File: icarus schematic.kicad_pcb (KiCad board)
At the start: 2 copper layers, 40 x 60 mm, 58 parts, among them J1 Conn_01x02_Socket, J2 USB_C_Receptacle_USB2.0_16P, J3 Conn_01x02_Socket, J4 Conn_01x02_Socket, J5 Conn_01x02_Socket, Q1 AO3400A, Q2 AO3400A, Q3 AO3400A, Q4 AO3400A, SW1 SW_Push(BOOt), SW2 SW_Push(EN), U2 BMI088, U3 AMS1117-3.3, U4 ESP32-S3-WROOM-1

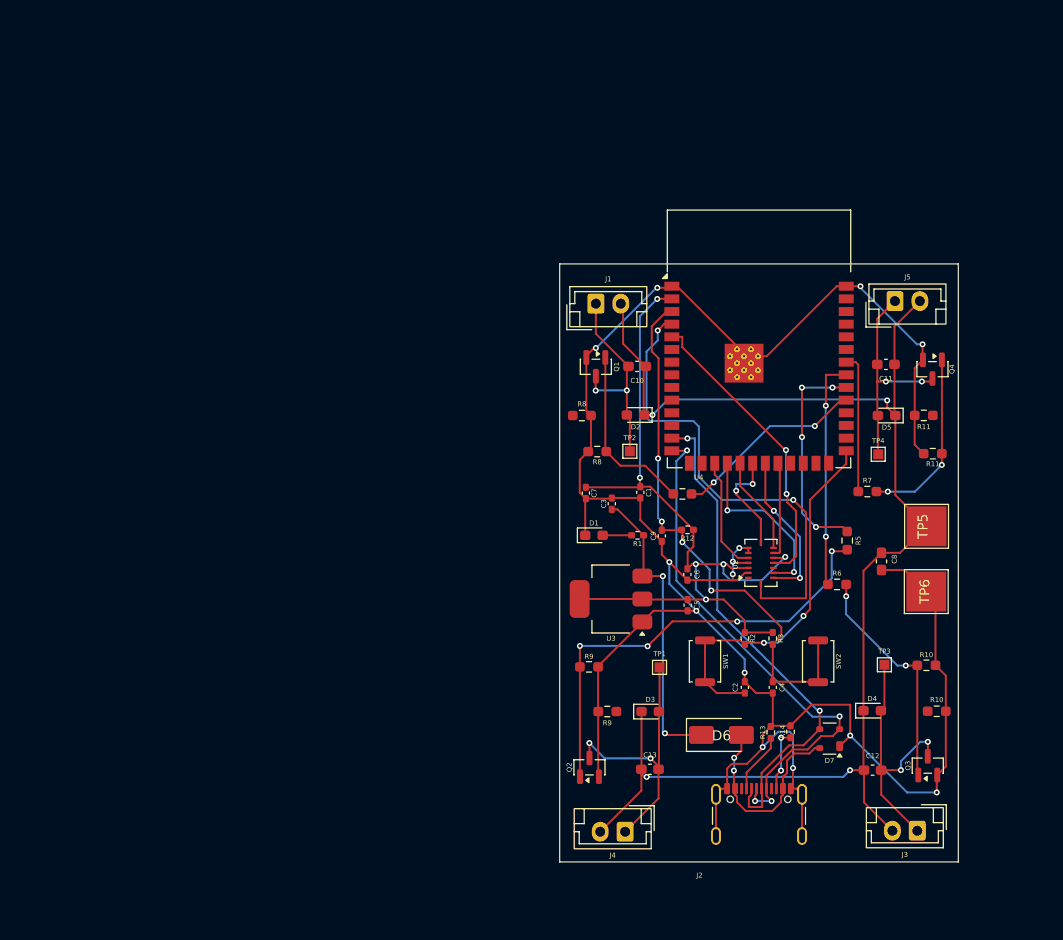
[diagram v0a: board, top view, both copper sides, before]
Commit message: Add files via upload
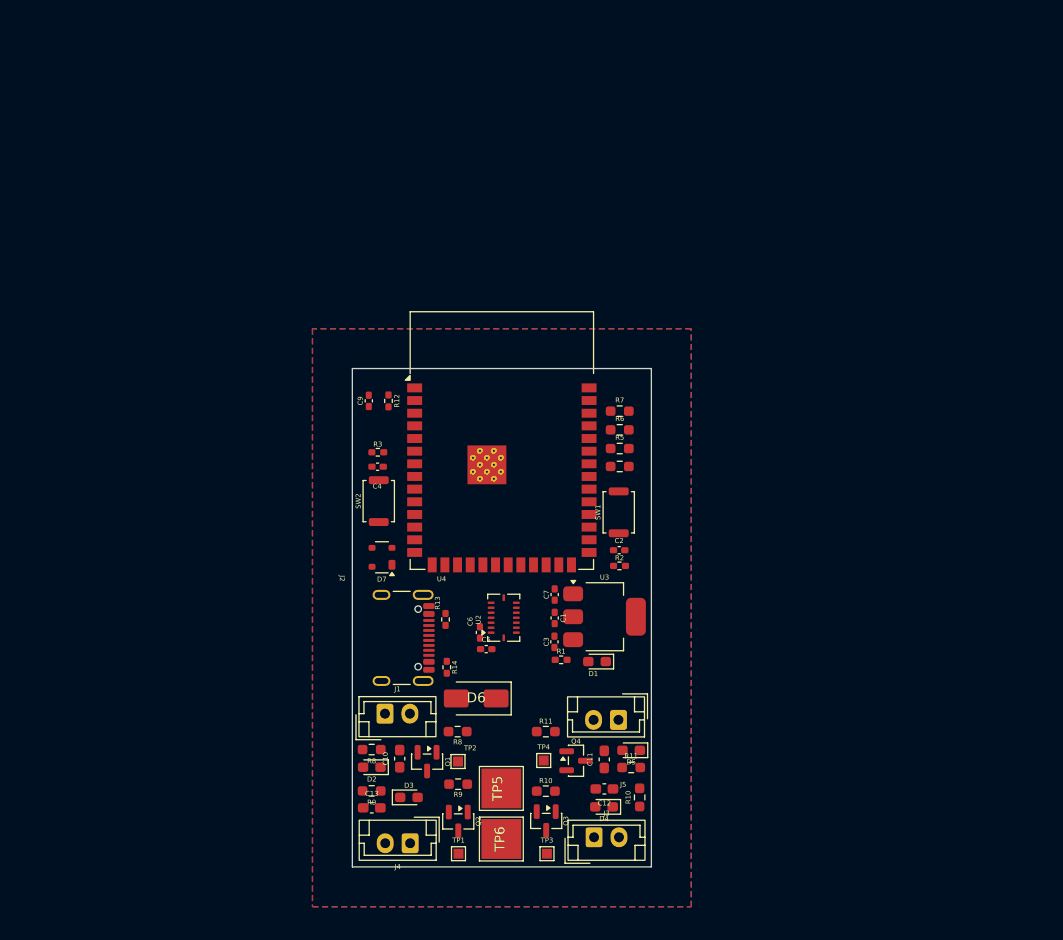
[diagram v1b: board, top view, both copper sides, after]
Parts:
- removed C8: 470uF, Capacitor_SMD:C_0603_1608Metric_Pad1.08x0.95mm_HandSolder
- moved Q4 53.1 mm to (129.4, 132.3), turned to 0 degrees
- moved J5 50.4 mm to (133.7, 128.2), turned to 180 degrees
- moved TP5 50.1 mm to (122.0, 135.1)
- moved TP6 49.3 mm to (122.0, 140.2)
- moved C11 48.7 mm to (132.3, 132.2), turned to 90 degrees
- moved D7 48.5 mm to (110.0, 111.9)
- moved R11 47.8 mm to (126.4, 129.4), turned to 0 degrees
- moved SW2 46.9 mm to (109.7, 106.3), turned to 90 degrees
- moved J1 46.3 mm to (110.3, 127.6)
- moved C10 46.0 mm to (111.8, 132.1), turned to 90 degrees
- moved R11 45.9 mm to (135.0, 133.0), turned to 0 degrees
- moved TP4 45.5 mm to (126.2, 132.3)
- moved C4 45.4 mm to (109.5, 102.8), turned to 180 degrees
- moved D2 44.2 mm to (109.0, 133.0)
- moved R3 43.8 mm to (109.6, 101.4), turned to 0 degrees
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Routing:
- net GND: track 228.0 -> 0.00 mm, vias 14 -> 0
- net Net-(D2-K): track 136.5 -> 0.00 mm, vias 4 -> 0
- net /3.3V: track 79.4 -> 0.00 mm, vias 6 -> 0
- net /EN: track 56.0 -> 0.00 mm, vias 4 -> 0
- net /USB_D+: track 53.4 -> 0.00 mm, vias 4 -> 0
- net /USB_D-: track 51.2 -> 0.00 mm, vias 2 -> 0
- net /INT1: track 48.5 -> 0.00 mm, vias 2 -> 0
- net /M2: track 45.6 -> 0.00 mm, vias 4 -> 0
- net /BOOT: track 38.3 -> 0.00 mm, vias 2 -> 0
- net /INT3: track 30.7 -> 0.00 mm, vias 2 -> 0
- net /5V: track 30.1 -> 0.00 mm, vias 2 -> 0
- net Net-(D3-A): track 27.6 -> 0.00 mm, vias 2 -> 0
- net Net-(D4-A): track 26.1 -> 0.00 mm, vias 2 -> 0
- net /M3: track 23.3 -> 0.00 mm, vias 2 -> 0
- net Net-(U4-IO40): track 23.2 -> 0.00 mm, vias 2 -> 0
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- added copper zone on B.Cu, net GND
- added copper zone on F.Cu, net GND
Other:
- board size 40 x 60 mm -> 30 x 50 mm

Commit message: Add files via upload
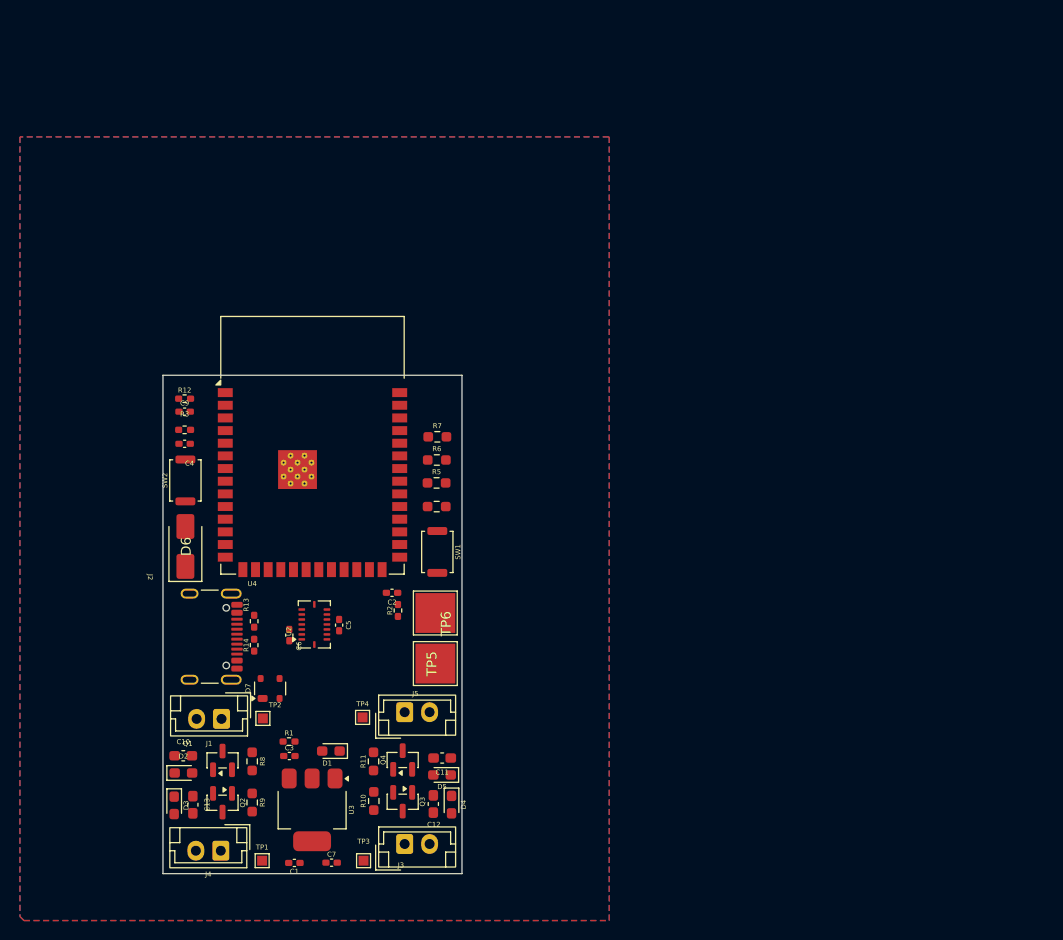
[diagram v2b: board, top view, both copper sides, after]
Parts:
- removed the R10 at (135.8, 136.0)
- removed the R11 at (135.0, 133.0)
- removed the R8 at (108.9, 131.2)
- removed the R9 at (108.9, 135.4)
- moved C1 35.9 mm to (101.2, 142.6), turned to 180 degrees
- moved U3 35.2 mm to (103.0, 137.3), turned to -90 degrees
- moved C7 35.0 mm to (104.9, 142.6), turned to 0 degrees
- moved D6 32.9 mm to (90.2, 110.8), turned to 90 degrees
- moved C3 29.0 mm to (100.7, 131.9), turned to 0 degrees
- moved R1 28.5 mm to (100.6, 130.4)
- moved D1 28.2 mm to (104.8, 131.4)
- moved Q2 23.7 mm to (94.0, 136.6)
- moved TP6 23.6 mm to (115.3, 117.5)
- moved D3 23.6 mm to (89.1, 136.8), turned to -90 degrees
- moved C2 23.2 mm to (111.0, 115.5), turned to 180 degrees
- moved R2 22.7 mm to (111.6, 117.3), turned to 90 degrees
- moved C10 21.7 mm to (90.0, 131.8), turned to 0 degrees
- moved J5 21.5 mm to (112.2, 127.5), turned to 0 degrees
- moved R8 20.8 mm to (97.0, 132.4), turned to -90 degrees
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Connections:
- SW1 pad 1: /BOOT -> GND
- SW2 pad 1: /EN -> GND

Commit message: Icarus PCB mk7 **finalised**
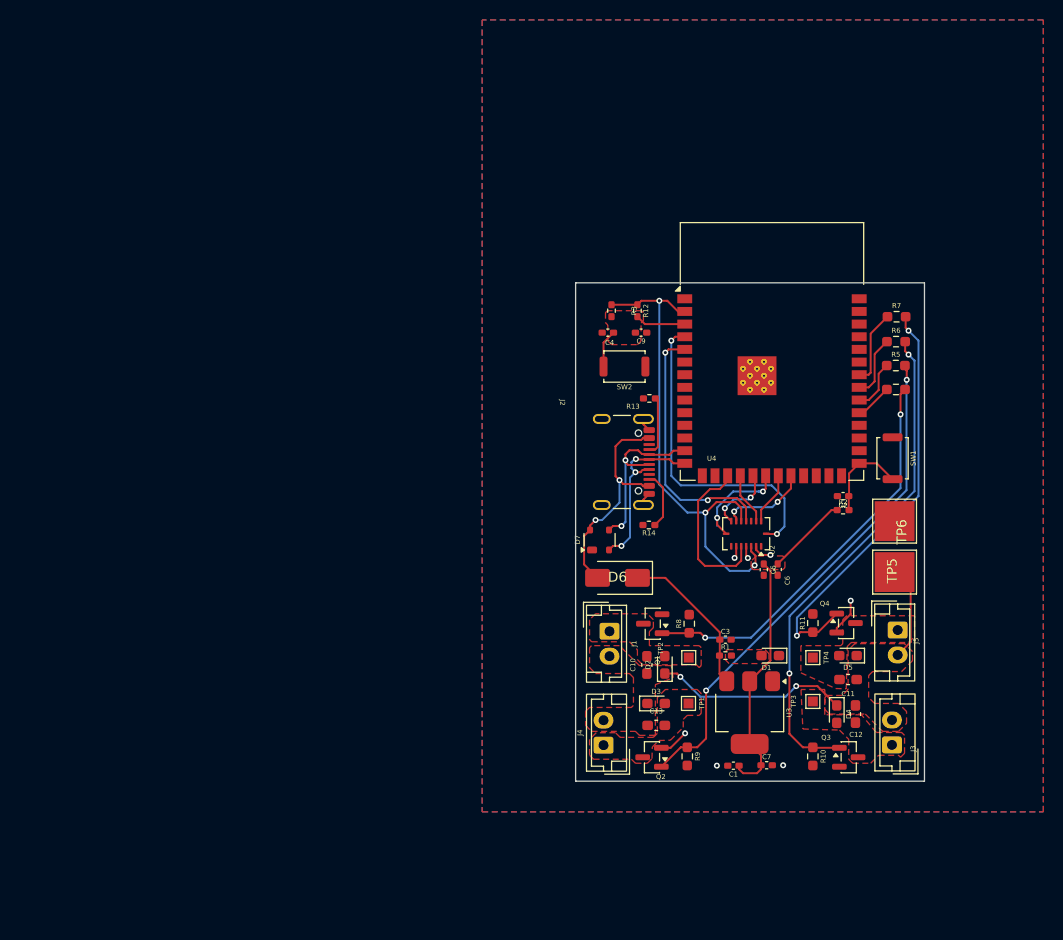
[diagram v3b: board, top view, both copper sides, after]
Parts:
- moved J5 50.1 mm to (161.7, 119.2), turned to -90 degrees
- moved J3 49.9 mm to (161.1, 130.8), turned to 90 degrees
- moved D2 49.5 mm to (138.3, 122.7), turned to 90 degrees
- moved C6 49.4 mm to (149.7, 113.2)
- moved D3 49.4 mm to (137.5, 126.6), turned to 0 degrees
- moved TP3 47.8 mm to (153.2, 126.4), turned to 90 degrees
- moved R7 47.6 mm to (161.6, 87.8)
- moved R6 47.6 mm to (161.6, 90.3)
- moved R5 47.6 mm to (161.5, 92.7)
- moved R4 47.5 mm to (161.5, 95.1)
- moved C10 47.4 mm to (136.6, 122.7), turned to 90 degrees
- moved C13 47.2 mm to (137.5, 128.8), turned to 0 degrees
- moved U4 47.1 mm to (149.1, 91.3)
- moved TP6 47.0 mm to (161.4, 108.3)
- moved TP5 47.0 mm to (161.4, 113.4)
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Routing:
- net /3.3V: track 0.00 -> 82.8 mm, vias 0 -> 3
- net /M2: track 0.00 -> 51.5 mm, vias 0 -> 2
- net /M3: track 0.00 -> 50.5 mm, vias 0 -> 2
- net /M4: track 0.00 -> 42.4 mm, vias 0 -> 2
- net /M1: track 0.00 -> 40.5 mm, vias 0 -> 2
- net /INT1: track 0.00 -> 32.3 mm, vias 0 -> 2
- net Net-(D2-K): track 0.00 -> 29.1 mm, vias 0 -> 2
- net /INT3: track 0.00 -> 26.0 mm, vias 0 -> 2
- net Net-(D6-A): track 0.00 -> 22.7 mm, vias 0 -> 2
- net /USB_D-: track 0.00 -> 18.0 mm, vias 0 -> 2
- net /USB_D+: track 0.00 -> 17.7 mm, vias 0 -> 3
- net /CSB2: track 0.00 -> 16.4 mm
- net /5V: track 0.00 -> 15.7 mm
- net GND: track 0.00 -> 14.0 mm, vias 0 -> 7
- net /SCK: track 0.00 -> 10.8 mm, vias 0 -> 2
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- added copper zone on F.Cu, net /3.3V
- added copper zone on F.Cu, net /EN
- added copper zone on F.Cu, net Net-(D1-A)
- added copper zone on F.Cu, net Net-(D2-A)
- added copper zone on F.Cu, net Net-(D2-K)
- added copper zone on F.Cu, net Net-(D3-A)
- added copper zone on F.Cu, net Net-(D4-A)
- added copper zone on F.Cu, net Net-(D5-A)
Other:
- board size 30 x 50 mm -> 35 x 50 mm
